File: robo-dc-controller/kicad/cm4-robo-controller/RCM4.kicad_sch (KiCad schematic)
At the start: 7 parts

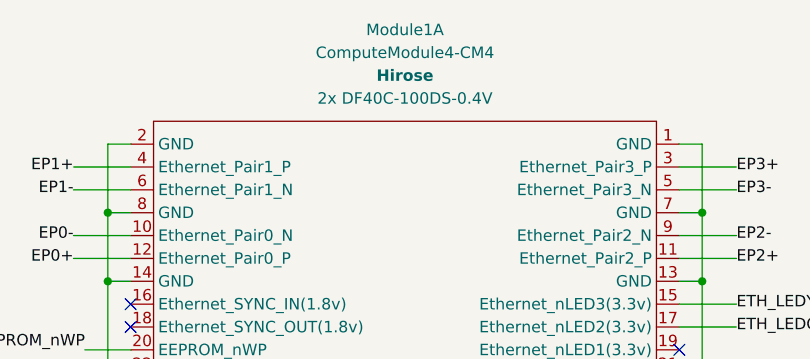
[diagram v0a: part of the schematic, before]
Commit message: Updates
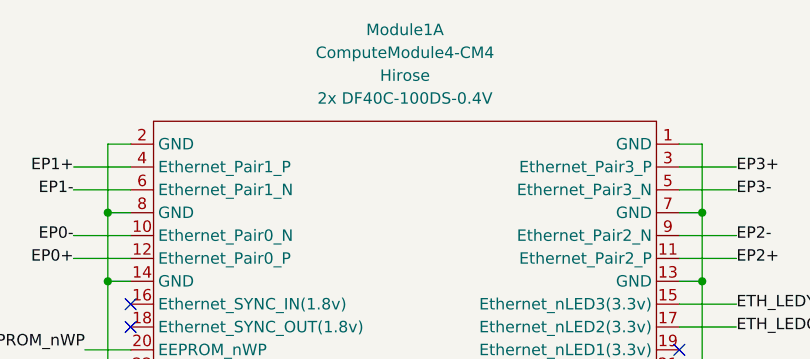
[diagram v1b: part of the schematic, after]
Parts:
- removed Module1: ComputeModule4-CM4, CM4_PARTS:Raspberry-Pi-4-Compute-Module, symbol CM4_Parts:ComputeModule4-CM4
- added Module1: ComputeModule4-CM4, CM4_PARTS:Raspberry-Pi-4-Compute-Module, symbol CM4Parts:ComputeModule4-CM4
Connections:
- net 1PPS_MCU: now also Module1.29 (GPIO16)
- net 3V3_CM4: now also Module1.78 (GPIO_VREF(1.8v/3.3v_Input)), Module1.84 (+3.3v_(Output)), Module1.86 (+3.3v_(Output))
- net 5V: now also Module1.77 (+5v_(Input)), Module1.79 (+5v_(Input)), Module1.81 (+5v_(Input)), Module1.83 (+5v_(Input)), Module1.85 (+5v_(Input)), Module1.87 (+5v_(Input))
- net AIN0: now also Module1.96 (AnalogIP0)
- net AIN1: now also Module1.94 (AnalogIP1)
- net BOOT_CONSOLE_RXD: now also Module1.51 (GPIO15)
- net BOOT_CONSOLE_TXD: now also Module1.55 (GPIO14)
- net EEPROM_nWP: now also Module1.20 (EEPROM_nWP)
- net EP0+: now also Module1.12 (Ethernet_Pair0_P)
- net EP0-: now also Module1.10 (Ethernet_Pair0_N)
- net EP1+: now also Module1.4 (Ethernet_Pair1_P)
- net EP1-: now also Module1.6 (Ethernet_Pair1_N)
- net EP2+: now also Module1.11 (Ethernet_Pair2_P)
- net EP2-: now also Module1.9 (Ethernet_Pair2_N)
- net EP3+: now also Module1.3 (Ethernet_Pair3_P)
- net EP3-: now also Module1.5 (Ethernet_Pair3_N)
- net ETH_LEDG: now also Module1.17 (Ethernet_nLED2(3.3v))
- net ETH_LEDY: now also Module1.15 (Ethernet_nLED3(3.3v))
- net GLOBAL_EN: now also Module1.99 (Global_EN)
- net GND: now also Module1.1 (GND), Module1.107 (GND), Module1.108 (GND), Module1.113 (GND), Module1.114 (GND), Module1.119 (GND), Module1.120 (GND), Module1.125 (GND), Module1.126 (GND), Module1.13 (GND), Module1.131 (GND), Module1.132 (GND), Module1.137 (GND), Module1.138 (GND), Module1.14 (GND), Module1.144 (GND), Module1.150 (GND), Module1.155 (GND), Module1.156 (GND), Module1.161 (GND), Module1.162 (GND), Module1.167 (GND), Module1.168 (GND), Module1.173 (GND), Module1.174 (GND), Module1.179 (GND), Module1.180 (GND), Module1.185 (GND), Module1.186 (GND), Module1.191 (GND), Module1.192 (GND), Module1.197 (GND), Module1.198 (GND), Module1.2 (GND), Module1.22 (GND), Module1.23 (GND), Module1.32 (GND), Module1.33 (GND), Module1.42 (GND), Module1.43 (GND), Module1.52 (GND), Module1.53 (GND), Module1.59 (GND), Module1.60 (GND), Module1.65 (GND), Module1.66 (GND), Module1.7 (GND), Module1.71 (GND), Module1.74 (GND), Module1.8 (GND), Module1.98 (GND)
- net GPIO22: now also Module1.46 (GPIO22)
- net I2C1_SCL: now also Module1.56 (GPIO3)
- net I2C1_SDA: now also Module1.58 (GPIO2)
- net PGOOD_12V: now also Module1.41 (GPIO25)
- net PWM0: now also Module1.31 (GPIO12)
- net PWM1: now also Module1.28 (GPIO13)
- net RUN_PG: now also Module1.92 (RUN_PG)
- net SPI0_CE0: now also Module1.39 (GPIO8)
- net SPI0_CE1: now also Module1.37 (GPIO7)
- net SPI0_MISO: now also Module1.40 (GPIO9)
- net SPI0_MOSI: now also Module1.44 (GPIO10)
- net SPI0_SCLK: now also Module1.38 (GPIO11)
- net USB2_N: now also Module1.103 (USB2_N)
- net USB2_P: now also Module1.105 (USB2_P)
- net USB_OTG_ID: now also Module1.101 (USB_OTG_ID)
- net nEXTRST: now also Module1.100 (nEXTRST)
- net nPWR_LED: now also Module1.95 (nPI_LED_PWR)
- net nRPIBOOT: now also Module1.93 (nRPIBOOT)
- net ~{FLT}: now also Module1.45 (GPIO24)
- net at R5.2: now also Module1.21 (PI_nLED_Activity)
- net at R2.2: now also Module1.30 (GPIO6)
- net at R3.2: now also Module1.34 (GPIO5)
- net at R4.2: now also Module1.54 (GPIO4)
